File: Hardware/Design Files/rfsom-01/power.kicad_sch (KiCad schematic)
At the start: 32 parts, among them U1 TPS62086RLT, U2 TPS51200DRCR, U3 LP8758A1E0YFFR

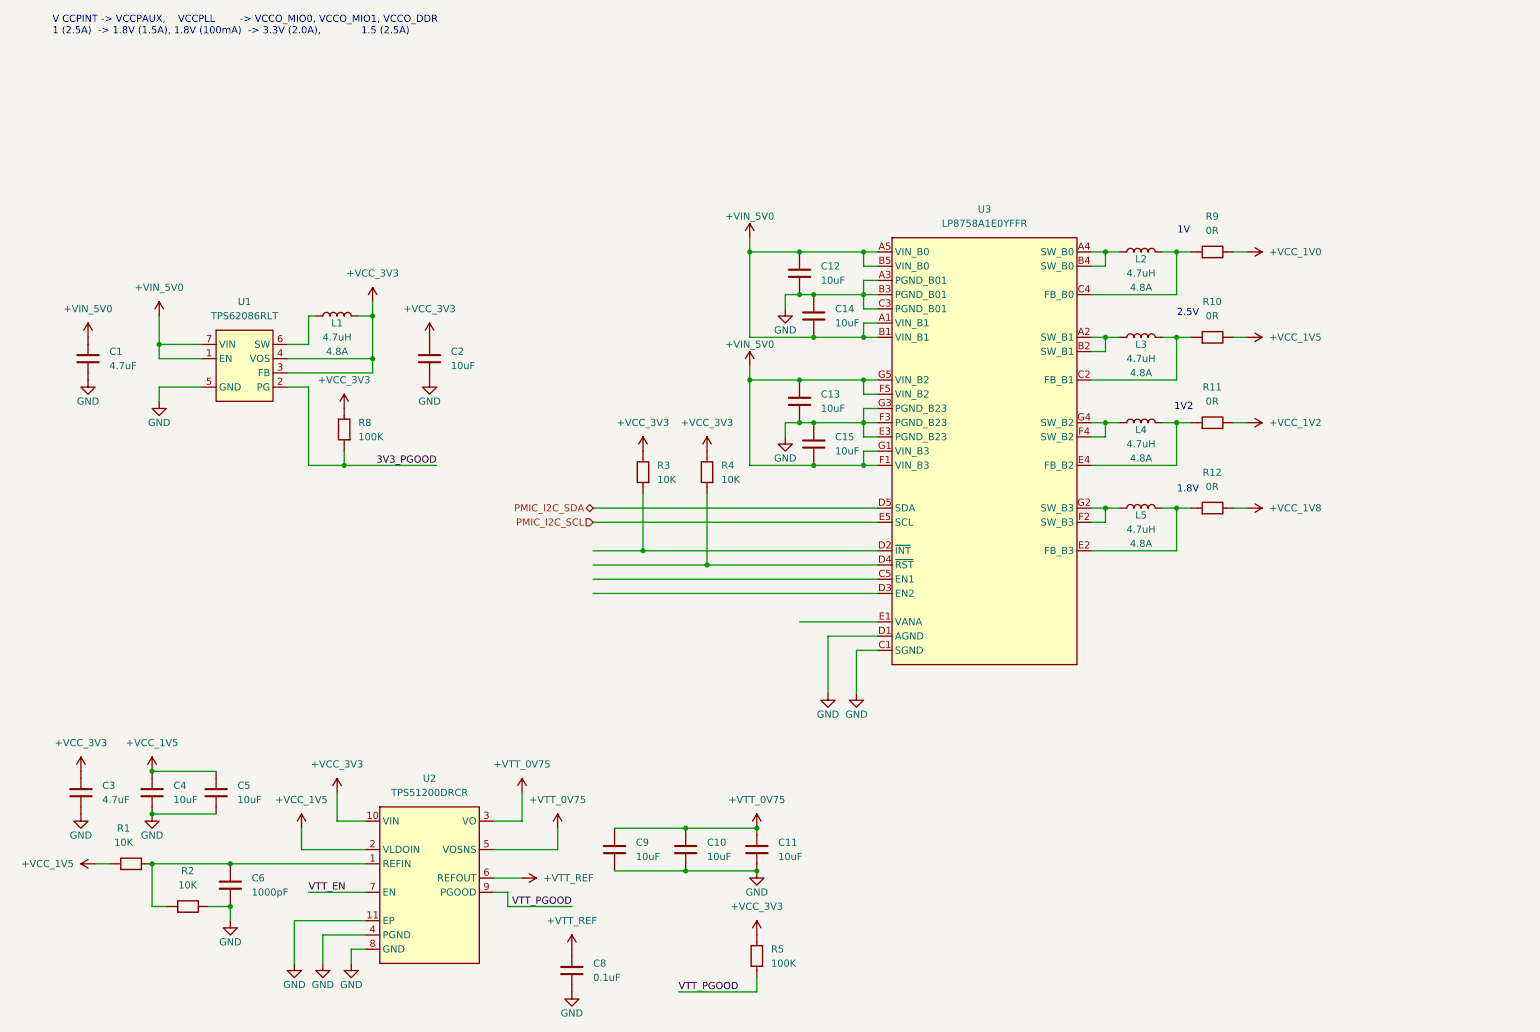
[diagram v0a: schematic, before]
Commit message: added starage, usb sch; more design progress in sch;
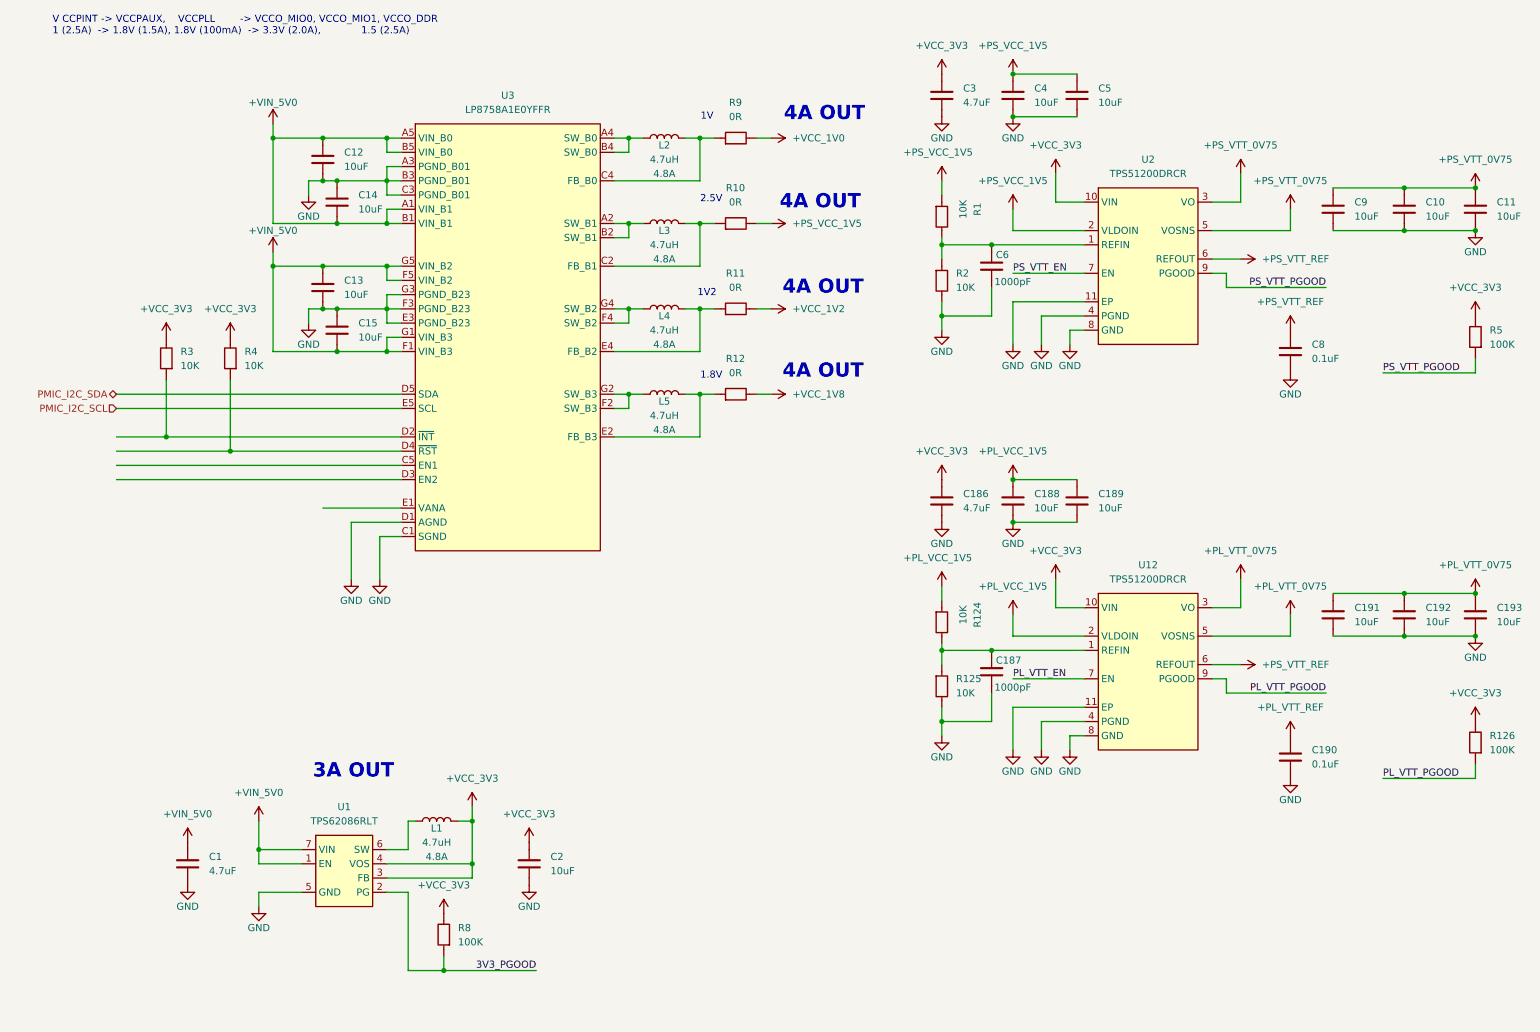
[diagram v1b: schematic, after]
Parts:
- added C186: CL21B475KPFNNNE, Capacitor_SMD:C_0805_2012Metric, symbol Capacitors:CL21B475KPFNNNE
- added C187: CL05B102KB5NNNC, Capacitor_SMD:C_0402_1005Metric, symbol Capacitors:CL05B102KB5NNNC
- added C188, C189, C191, C192, C193: CL21B106KQQNFNE, Capacitor_SMD:C_0805_2012Metric, symbol Capacitors:CL21B106KQQNFNE
- added C190: CL05B104KA5NNNC, Capacitor_SMD:C_0402_1005Metric, symbol Capacitors:CL05B104KA5NNNC
- added R124, R125: RC0603FR-0710KL, Resistor_SMD:R_0603_1608Metric, symbol Resistors:RC0603FR-0710KL
- added R126: RC0402FR-07100KL, Resistor_SMD:R_0402_1005Metric, symbol Resistors:RC0402FR-07100KL
- added U12: TPS51200DRCR, Package_SON:VSON-10-1EP_3x3mm_P0.5mm_EP1.65x2.4mm, symbol ICs:TPS51200DRCR
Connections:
- net +VCC_3V3: now also C186.1, R126.2, U12.10 (VIN)
- net GND: now also C186.2, C187.2, C188.2, C189.2, C190.2, C191.2, C192.2, C193.2, R125.2, U12.11 (EP), U12.4 (PGND), U12.8 (GND)
- net +VCC_1V5 renamed +PS_VCC_1V5
- net +VTT_0V75 renamed +PS_VTT_0V75
- net +VTT_REF renamed +PS_VTT_REF
- net +PS_VTT_REF: now also U12.6 (REFOUT)
- net VTT_EN renamed PS_VTT_EN
- net VTT_PGOOD renamed PS_VTT_PGOOD
- new net: C187.1, R124.2, R125.1, U12.1 (REFIN)
- new net +PL_VCC_1V5: C188.1, C189.1, R124.1, U12.2 (VLDOIN)
- new net +PL_VTT_0V75: C191.1, C192.1, C193.1, U12.3 (VO), U12.5 (VOSNS)
- new net +PL_VTT_REF: C190.1
- new net PL_VTT_EN: U12.7 (EN)
- new net PL_VTT_PGOOD: R126.1, U12.9 (PGOOD)
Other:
- note added: "3A OUT"
- note added: "4A OUT"
- moved on the sheet: C1, C10, C11, C12, C13, C14, C15, C2, C3, C4, C5, C6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
